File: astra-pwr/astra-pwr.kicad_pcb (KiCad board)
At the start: 2 copper layers, 45 parts, among them J1 12V_IN, J2 RPI_PWR, J3 MISC_OUT, J4 STATUS_LED, U1 LMR54410DBVR, U2 TPS563240DDC, U3 LM321MF, U4 LM321MF, U5 LM321MF

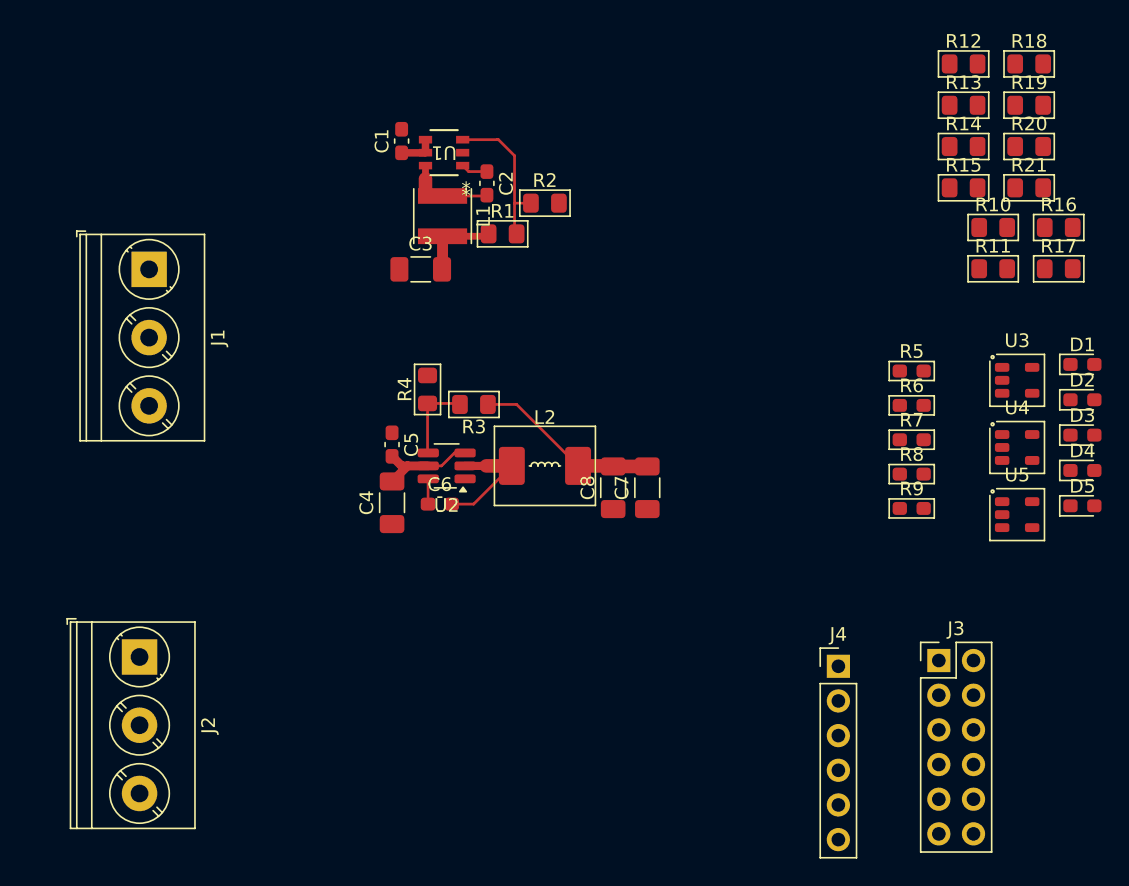
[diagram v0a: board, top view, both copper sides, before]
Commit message: Finished first iteration of power board
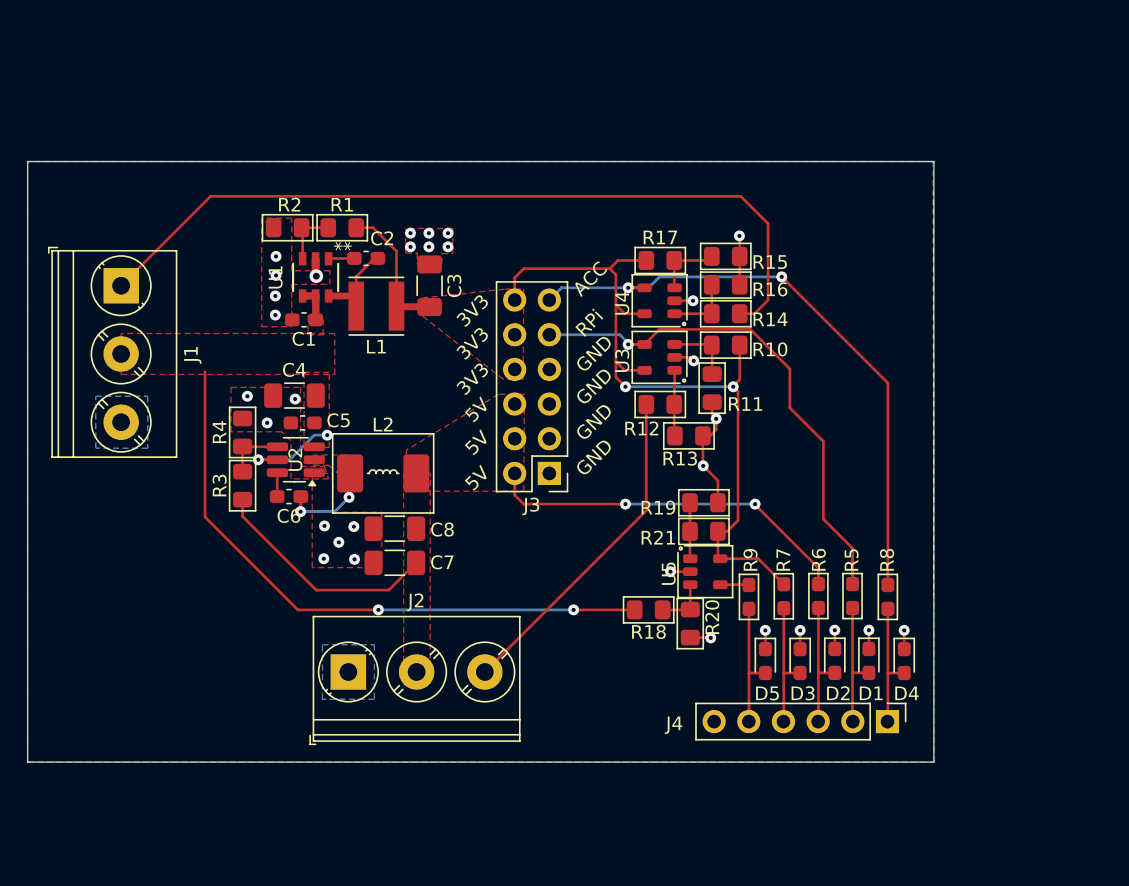
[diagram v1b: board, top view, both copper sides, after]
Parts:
- moved R18 48.8 mm to (83.1, 72.0), turned to 180 degrees
- moved R20 42.9 mm to (86.2, 73.0), turned to -90 degrees
- moved R19 37.6 mm to (87.2, 64.2)
- moved R21 34.7 mm to (87.2, 66.3), turned to 180 degrees
- moved R12 33.4 mm to (84.0, 57.0)
- moved J3 31.7 mm to (75.8, 62.0), turned to 180 degrees
- moved R13 31.5 mm to (86.0, 59.3), turned to 180 degrees
- moved R17 29.2 mm to (84.0, 46.5)
- moved U4 28.3 mm to (83.9, 49.4), turned to 180 degrees
- moved D1 26.8 mm to (99.2, 75.8), turned to -90 degrees
- moved D3 26.5 mm to (94.2, 75.8), turned to -90 degrees
- moved D2 26.4 mm to (96.7, 75.8), turned to -90 degrees
- moved U3 26.3 mm to (83.9, 53.5), turned to 180 degrees
- moved D5 25.9 mm to (91.7, 75.8), turned to -90 degrees
- moved R16 24.8 mm to (88.8, 48.2), turned to 180 degrees
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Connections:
- J2 pad 1: 5V -> GND
- J2 pad 2: RPI_5V -> 5V
- J2 pad 3: GND -> RPI_5V
- J3 pad 1: RPI_PWR -> GND
- J3 pad 10: 5V -> 3V3
- J3 pad 11: GND -> ACC_UP
- J3 pad 12: 5V -> 3V3
- J3 pad 2: 3V3 -> 5V
- J3 pad 3: ACC_UP -> GND
- J3 pad 4: 3V3 -> 5V
- J3 pad 6: 3V3 -> 5V
- J3 pad 8: 5V -> 3V3
- J3 pad 9: GND -> RPI_PWR
- J4 pad 1: RPI_PWR_IND -> ACC_UP_IND
- J4 pad 2: 5V_IND -> RPI_PWR_IND
- J4 pad 3: 3V3_IND -> 5V_IND
- J4 pad 4: ACC_UP_IND -> 3V3_IND
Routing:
- net 3V3: track 5.31 -> 66.2 mm, vias 0 -> 2
- net ACC: track 0.00 -> 59.0 mm
- net ACC_UP: track 0.00 -> 44.9 mm, vias 0 -> 2
- net BAT: track 10.5 -> 55.0 mm, vias 0 -> 4
- net RPI_PWR: track 0.00 -> 37.2 mm, vias 0 -> 1
- net 5V: track 13.6 -> 44.3 mm, vias 0 -> 2
- net GND: track 0.00 -> 26.7 mm, vias 0 -> 31
- net RPI_5V: track 0.00 -> 24.5 mm
- net 5V_IND: track 0.00 -> 9.54 mm
- net 3V3_IND: track 0.00 -> 9.53 mm
- net ACC_UP_IND: track 0.00 -> 9.48 mm
- net BAT_LOW_IND: track 0.00 -> 9.47 mm
- net RPI_PWR_IND: track 0.00 -> 9.17 mm
- net 3V3_FB: track 11.2 -> 4.26 mm
- net Net-(U3--): track 0.00 -> 5.16 mm
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- added copper zone on F.Cu, net 3V3
- added copper zone on F.Cu, net 5V
- added copper zone on F.Cu, net BAT
- added copper zone on B.Cu, net GND
- added copper zone on F.Cu, net GND
- added copper zone on F.Cu, net Net-(U2-SW)
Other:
- board outline added: 66.4 x 44 mm
- board text added: "3V3"
- board text added: "5V"
- board text added: "ACC"
- board text added: "GND"
- board text added: "RPi"
